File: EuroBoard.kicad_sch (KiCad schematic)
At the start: 35 parts, among them J1 GPIO, J10 PD1, J11 PD2, J12 PD3, J2 Conn_01x07_Male, J3 I2C, J4 Conn_01x05_Male, J5 RX, J6 TX, J7 GND, SW1 RESET, SW2 SW_DIP_x04, U1 AMS1117-3.3, U2 STM32G030CxT, Y1 NX2520 16MHz

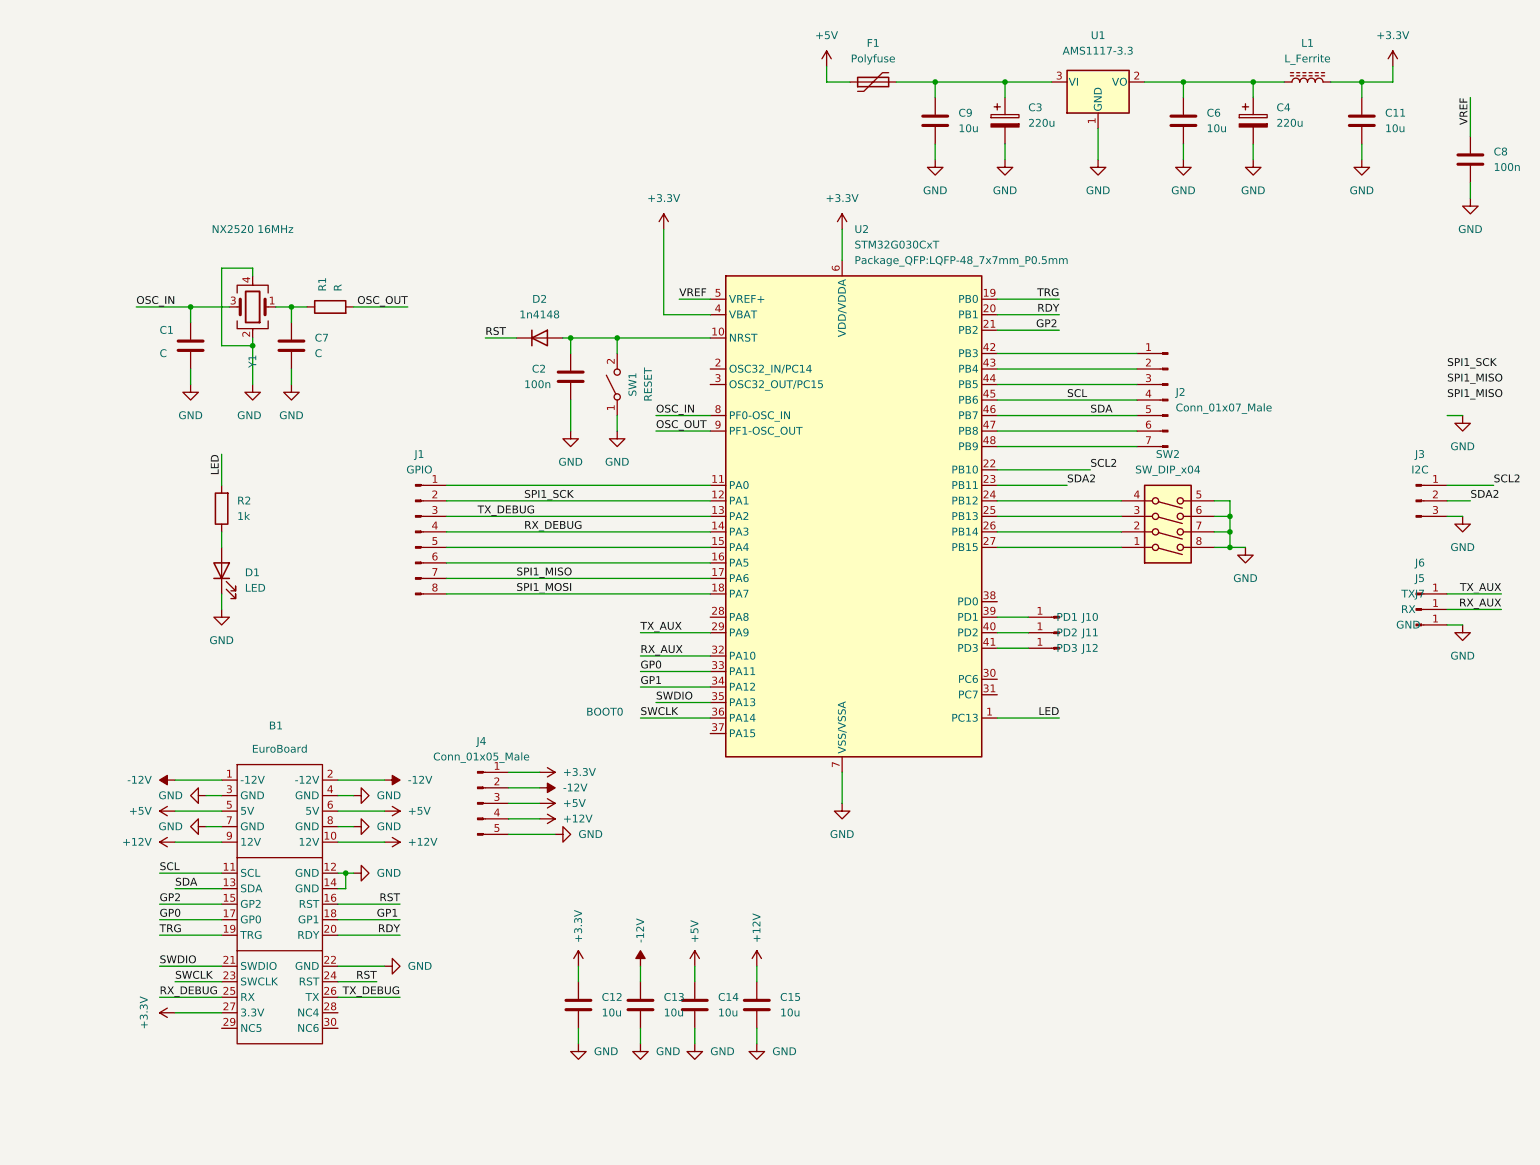
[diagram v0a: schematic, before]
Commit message: Rework
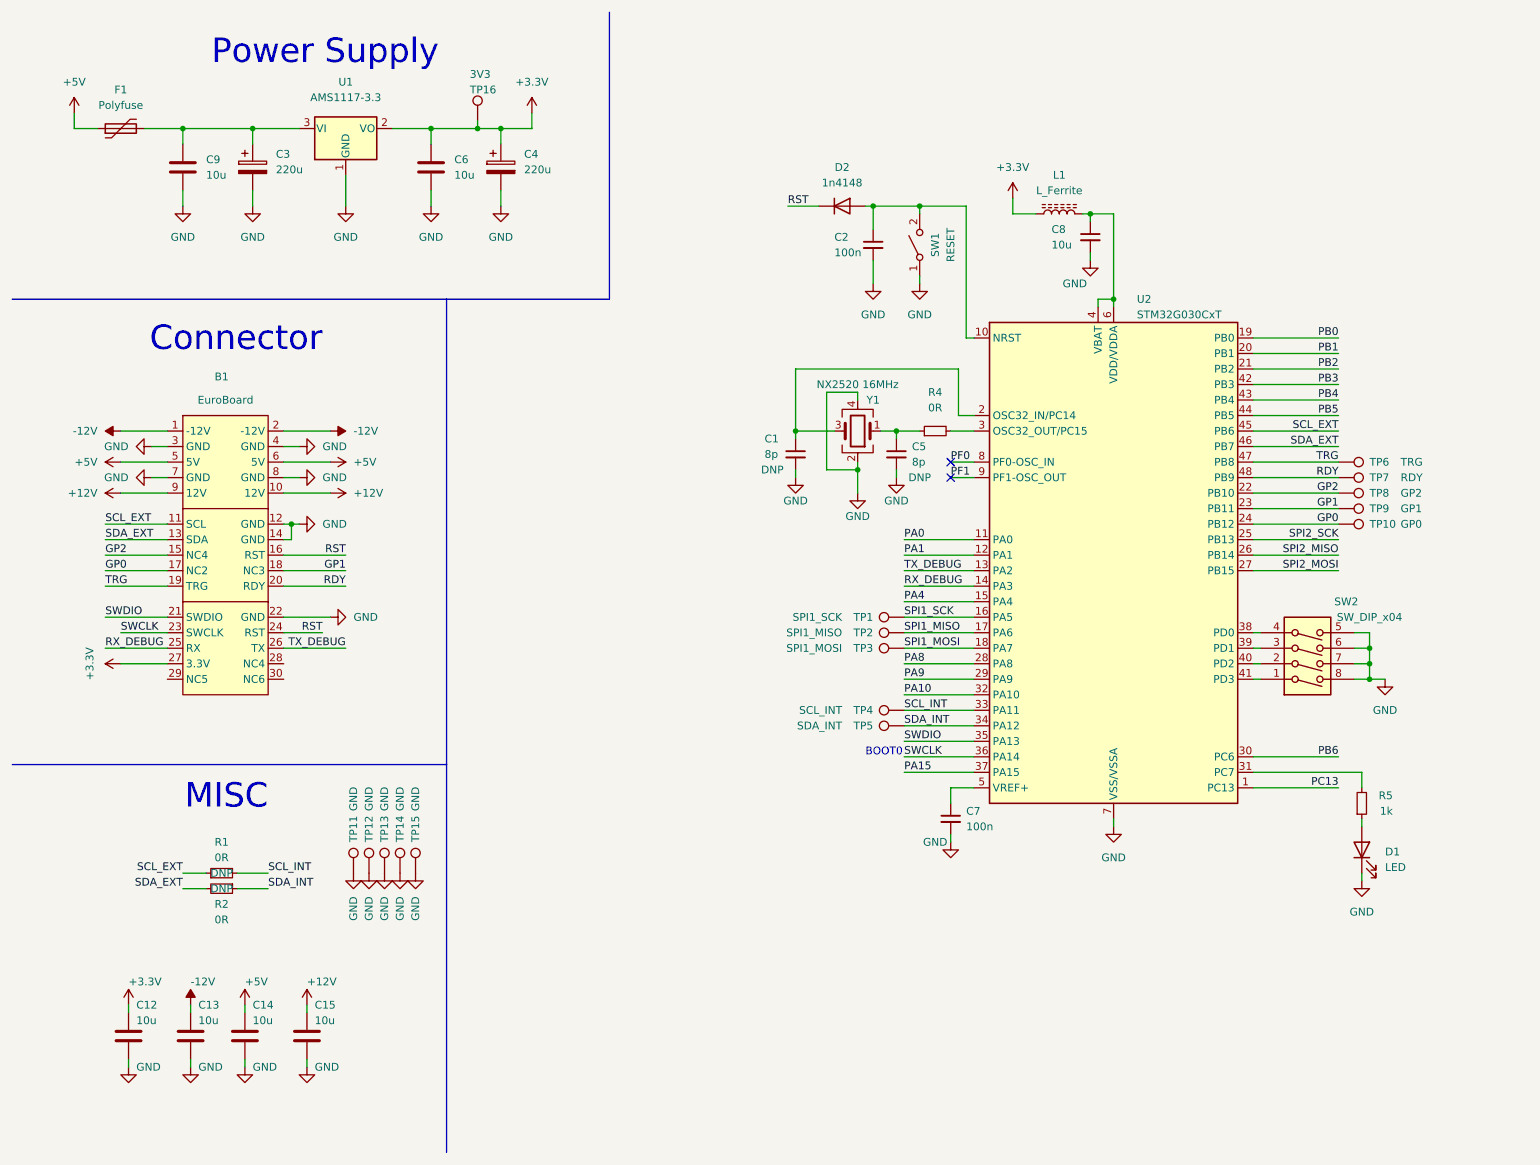
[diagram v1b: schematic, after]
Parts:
- removed C1, C7: C, Capacitor_SMD:C_0805_2012Metric_Pad1.18x1.45mm_HandSolder, symbol Device:C
- removed C11: 10u, Capacitor_SMD:C_0805_2012Metric_Pad1.18x1.45mm_HandSolder, symbol Device:C
- removed C2, C8: 100n, Capacitor_SMD:C_0805_2012Metric_Pad1.18x1.45mm_HandSolder, symbol Device:C
- removed J1: GPIO, Connector_PinHeader_2.54mm:PinHeader_1x08_P2.54mm_Vertical, symbol Connector:Conn_01x08_Male
- removed J10: PD1, TestPoint:TestPoint_Pad_1.0x1.0mm, symbol Connector:Conn_01x01_Male
- removed J11: PD2, TestPoint:TestPoint_Pad_1.0x1.0mm, symbol Connector:Conn_01x01_Male
- removed J12: PD3, TestPoint:TestPoint_Pad_1.0x1.0mm, symbol Connector:Conn_01x01_Male
- removed J2: Conn_01x07_Male, Connector_PinHeader_2.54mm:PinHeader_1x07_P2.54mm_Vertical, symbol Connector:Conn_01x07_Male
- removed J3: I2C, Connector_PinHeader_2.54mm:PinHeader_1x03_P2.54mm_Vertical, symbol Connector:Conn_01x03_Male
- removed J4: Conn_01x05_Male, Connector_PinHeader_2.54mm:PinHeader_1x05_P2.54mm_Vertical, symbol Connector:Conn_01x05_Male
- removed J5: RX, TestPoint:TestPoint_Pad_1.0x1.0mm, symbol Connector:Conn_01x01_Male
- removed J6: TX, TestPoint:TestPoint_Pad_1.0x1.0mm, symbol Connector:Conn_01x01_Male
- removed J7: GND, TestPoint:TestPoint_Pad_1.0x1.0mm, symbol Connector:Conn_01x01_Male
- removed R1: R, Resistor_SMD:R_0805_2012Metric_Pad1.20x1.40mm_HandSolder, symbol Device:R
- removed R2: 1k, Resistor_SMD:R_0805_2012Metric_Pad1.20x1.40mm_HandSolder, symbol Device:R
- added C1, C5: 8p, Capacitor_SMD:C_0805_2012Metric_Pad1.18x1.45mm_HandSolder, symbol Device:C_Small
- added C2, C7: 100n, Capacitor_SMD:C_0805_2012Metric_Pad1.18x1.45mm_HandSolder, symbol Device:C_Small
- added C8: 10u, Capacitor_SMD:C_0805_2012Metric_Pad1.18x1.45mm_HandSolder, symbol Device:C_Small
- added R1, R2, R4: 0R, Capacitor_SMD:C_0805_2012Metric_Pad1.18x1.45mm_HandSolder, symbol Device:R_Small
- added R5: 1k, Resistor_SMD:R_0805_2012Metric_Pad1.20x1.40mm_HandSolder, symbol Device:R_Small
- added TP1: SPI1_SCK, MEMS_Custom:TestPoint_Pad_D1.0mm, symbol Connector:TestPoint
- added TP10: GP0, MEMS_Custom:TestPoint_Pad_D1.0mm, symbol Connector:TestPoint
- added TP11, TP12, TP13, TP14, TP15: GND, MEMS_Custom:TestPoint_Pad_D1.0mm, symbol Connector:TestPoint
- added TP16: 3V3, MEMS_Custom:TestPoint_Pad_D1.0mm, symbol Connector:TestPoint
- added TP2: SPI1_MISO, MEMS_Custom:TestPoint_Pad_D1.0mm, symbol Connector:TestPoint
- added TP3: SPI1_MOSI, MEMS_Custom:TestPoint_Pad_D1.0mm, symbol Connector:TestPoint
- added TP4: SCL_INT, MEMS_Custom:TestPoint_Pad_D1.0mm, symbol Connector:TestPoint
- added TP5: SDA_INT, MEMS_Custom:TestPoint_Pad_D1.0mm, symbol Connector:TestPoint
- added TP6: TRG, MEMS_Custom:TestPoint_Pad_D1.0mm, symbol Connector:TestPoint
- added TP7: RDY, MEMS_Custom:TestPoint_Pad_D1.0mm, symbol Connector:TestPoint
- added TP8: GP2, MEMS_Custom:TestPoint_Pad_D1.0mm, symbol Connector:TestPoint
- added TP9: GP1, MEMS_Custom:TestPoint_Pad_D1.0mm, symbol Connector:TestPoint
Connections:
- net SCL2 is gone; now on net GP2: U2.22 (PB10)
- net SDA2 is gone; now on net GP1: U2.23 (PB11)
- net +3.3V: now also C4.1, C6.1, L1.1, U1.2 (VO), TP16.1; no longer L1.2, U2.4 (VBAT), U2.6 (VDD/VDDA)
- net GND: now also C1.2, C2.2, C5.2, C7.2, C8.2, TP11.1, TP12.1, TP13.1, TP14.1, TP15.1
- net GP0: now also U2.24 (PB12), TP10.1; no longer U2.33 (PA11)
- net GP1: now also TP9.1; no longer U2.34 (PA12)
- net GP2: now also TP8.1; no longer U2.21 (PB2)
- net RDY: now also U2.48 (PB9), TP7.1; no longer U2.20 (PB1)
- net SPI1_MISO: now also TP2.1
- net SPI1_MOSI: now also TP3.1
- net SPI1_SCK: now also U2.16 (PA5), TP1.1; no longer U2.12 (PA1)
- net TRG: now also U2.47 (PB8), TP6.1; no longer U2.19 (PB0)
- net at D2.2 (A), SW1.2 (B), U2.10 (NRST): now also C2.1
- net PA0: now reaches U2.11 (PA0)
- net PA4: now reaches U2.15 (PA4)
- net at D1.2 (A): now also R5.1
- net at U2.2 (OSC32_IN/PC14): now also Y1.3, C1.1
- net at SW2.4: now also U2.38 (PD0); no longer U2.24 (PB12)
- net at SW2.3: now also U2.39 (PD1); no longer U2.25 (PB13)
- net at SW2.2: now also U2.40 (PD2); no longer U2.26 (PB14)
- net at SW2.1: now also U2.41 (PD3); no longer U2.27 (PB15)
- net PA8: now reaches U2.28 (PA8)
- net at U2.3 (OSC32_OUT/PC15): now also R4.2
- net PB6: now reaches U2.30 (PC6)
- net at U2.31 (PC7): now also R5.2
- net PA15: now reaches U2.37 (PA15)
- net PB3: now reaches U2.42 (PB3)
- net PB4: now reaches U2.43 (PB4)
- net PB5: now reaches U2.44 (PB5)
- net at Y1.1: now also C5.1, R4.1
- net LED renamed PC13
- net OSC_IN renamed PF0
- net PF0: no longer Y1.3
- net OSC_OUT renamed PF1
- net RX_AUX renamed PA10
- net SCL renamed SCL_EXT
- net SCL_EXT: now also R1.1
- net SDA renamed SDA_EXT
- net SDA_EXT: now also R2.2
- net TX_AUX renamed PA9
- net VREF: no longer names the net of U2.5 (VREF+)
- net VREF: now also C7.1
- new net: C8.1, L1.2, U2.4 (VBAT), U2.6 (VDD/VDDA)
- new net PA1: U2.12 (PA1)
- new net PB0: U2.19 (PB0)
- new net PB1: U2.20 (PB1)
- new net PB2: U2.21 (PB2)
- new net SCL_INT: R1.2, TP4.1, U2.33 (PA11)
- new net SDA_INT: R2.1, TP5.1, U2.34 (PA12)
- new net SPI2_MISO: U2.26 (PB14)
- new net SPI2_MOSI: U2.27 (PB15)
- new net SPI2_SCK: U2.25 (PB13)
- no-connect marks 0 -> 2
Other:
- note added: "Connector"
- note added: "MISC"
- note added: "Power Supply"
- title: (none) -> EuroMeasure-Module
- moved on the sheet: C12, C13, C14, C15, C3, C4, C6, C9, D1, D2, F1, L1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
